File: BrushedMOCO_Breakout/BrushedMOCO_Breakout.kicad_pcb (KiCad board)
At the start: 2 copper layers, 39.9 x 46.2 mm, 30 parts, among them Q1 Si4156DY, Q2 Si4156DY, Q3 Si4156DY, Q4 Si4156DY, U1 74LVC2G04, U2 IRS2308, U3 IRS2308

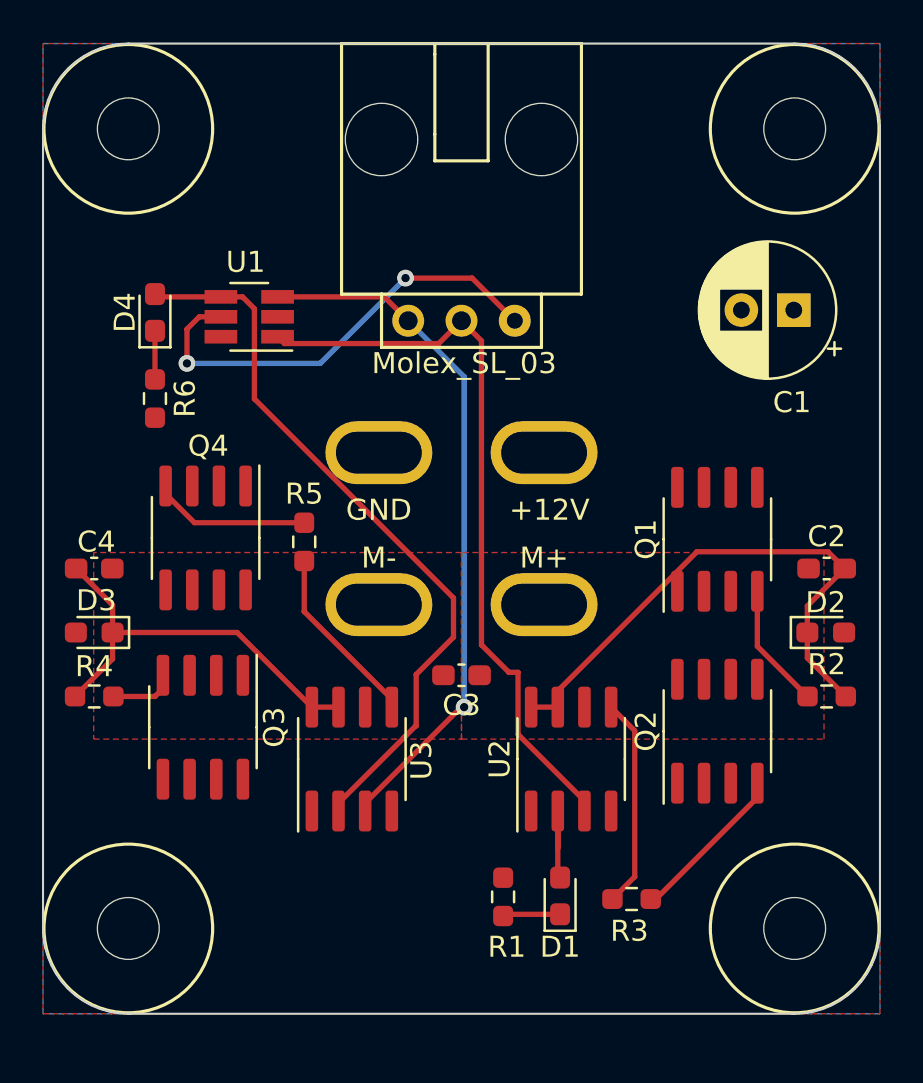
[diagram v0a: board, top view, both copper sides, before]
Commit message: Finish layout for order
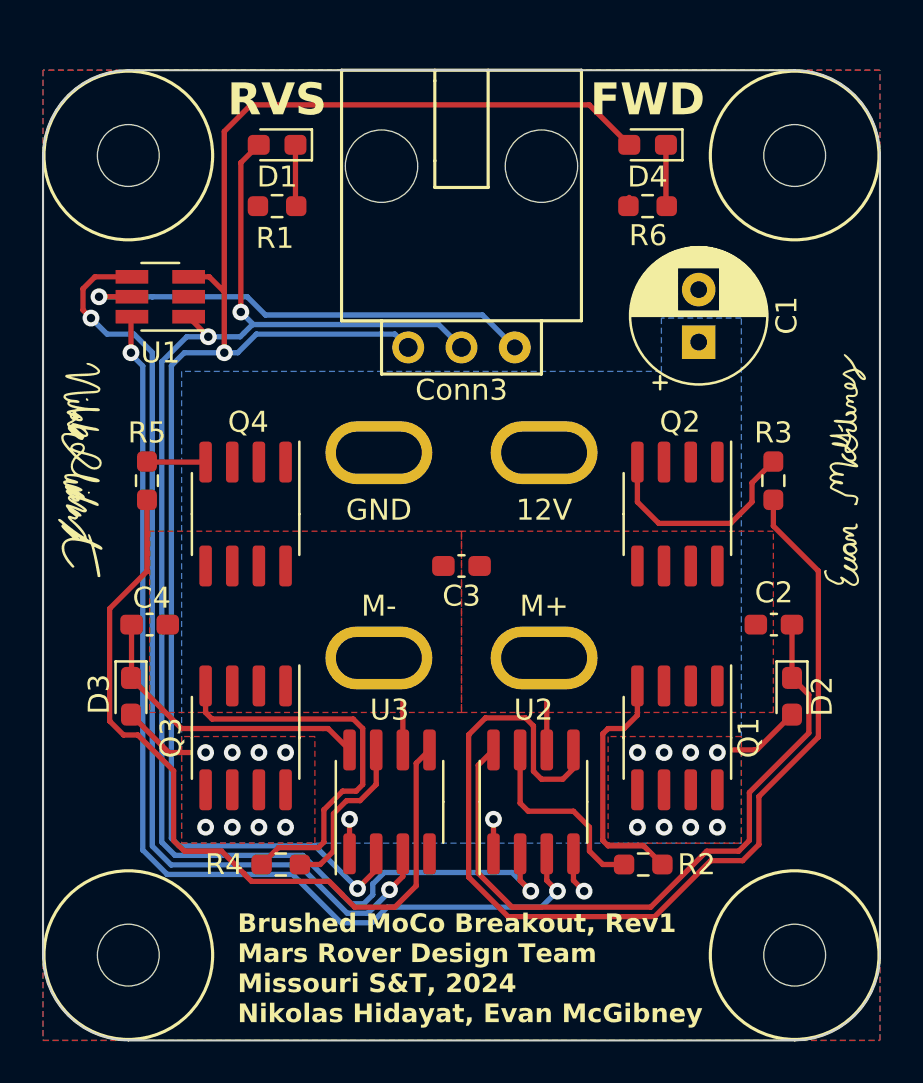
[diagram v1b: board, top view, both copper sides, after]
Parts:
- G*** (x2): moved to F.Cu
- R1, R6: value 120 -> 100
- moved D1 38.2 mm to (112.8, 81.0), turned to 180 degrees
- moved R1 34.6 mm to (112.8, 83.9), turned to 180 degrees
- moved G*** 32.4 mm to (103.3, 96.7), turned to -90 degrees
- moved R6 25.2 mm to (130.4, 83.9), turned to 180 degrees
- moved D4 24.8 mm to (130.4, 81.0), turned to 180 degrees
- moved R3 21.0 mm to (136.4, 97.0), turned to 90 degrees
- moved G*** 12.5 mm to (139.8, 96.4)
- moved R4 12.0 mm to (112.9, 115.3), turned to 180 degrees
- moved R2 11.9 mm to (130.2, 115.3), turned to 0 degrees
- moved Q2 10.5 mm to (131.8, 98.6), turned to -90 degrees
- moved Q1 9.65 mm to (131.8, 109.3), turned to -90 degrees
- moved R5 8.04 mm to (106.6, 97.0)
- moved C3 5.21 mm to (121.5, 101.1)
- moved C1 4.78 mm to (132.8, 90.4), turned to 90 degrees
- moved U1 4.34 mm to (107.2, 88.3)
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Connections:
- C1 pad 1: GND -> +12V
- C1 pad 2: +12V -> GND
- D1 pad 2: Net-(D1-A) -> PWM_FWD
- D4 pad 2: Net-(D4-A) -> PWM_RVS
- R2 pad 1: Net-(D2-K) -> Net-(U2-HO)
- R4 pad 1: Net-(D3-K) -> Net-(U3-HO)
- U1 pad 4: Net-(D4-A) -> Net-(U3-LIN)
- U1 pad 6: Net-(D1-A) -> Net-(U2-LIN)
- U2 pad 2: Net-(D1-A) -> PWM_FWD
- U2 pad 3: PWM_FWD -> Net-(U2-LIN)
- U2 pad 7: Net-(D2-K) -> Net-(U2-HO)
- U3 pad 2: Net-(D4-A) -> PWM_RVS
- U3 pad 3: PWM_RVS -> Net-(U3-LIN)
- U3 pad 7: Net-(D3-K) -> Net-(U3-HO)
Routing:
- net Net-(U2-LIN): track 0.00 -> 49.5 mm, vias 0 -> 2
- net PWM_RVS: track 33.2 -> 79.7 mm, vias 1 -> 2
- net Net-(U3-LIN): track 0.00 -> 46.4 mm, vias 0 -> 2
- net Net-(U2-LO): track 10.1 -> 50.2 mm
- net PWM_FWD: track 35.4 -> 70.9 mm, vias 0 -> 3
- net Net-(D4-A): track 35.2 -> 0.00 mm
- net Net-(U3-LO): track 8.69 -> 38.7 mm
- net Net-(Q3-G): track 2.70 -> 19.0 mm
- net +12V: track 0.00 -> 10.3 mm, vias 0 -> 18
- net Net-(U2-HO): track 0.00 -> 9.37 mm
- net Net-(U3-HO): track 0.00 -> 8.93 mm
- net Net-(D2-K): track 26.4 -> 33.3 mm
- net Net-(Q1-G): track 5.31 -> 11.8 mm
- net Net-(D3-K): track 19.8 -> 14.4 mm
- net Net-(Q4-G): track 7.99 -> 2.80 mm
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- added copper zone on F.Cu, net +12V
- added copper zone on B.Cu, net GND
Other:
- board text added: "12V"
- board text added: "Brushed MoCo Breakout, Rev1 Mars Rover Design Team Missouri S&T, 2024 Nikolas Hidayat, Evan McGibney"
- board text added: "FWD"
- board text added: "RVS"
- board text removed: "+12V"
- board text removed: "BrushedMOCO Breakout, Rev1 Mars Rover Design Team Missouri S&T, 2024 Nikolas Hidayat, Evan McGibney"
- board text removed: "Molex_SL_03"
